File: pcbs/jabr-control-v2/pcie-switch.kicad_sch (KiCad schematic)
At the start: 27 parts, among them Q301 DMN21D2UFB-7B, U301 SYA75603A, U302 PCI11010C, Y301 XRCGB25M000F3A16R0

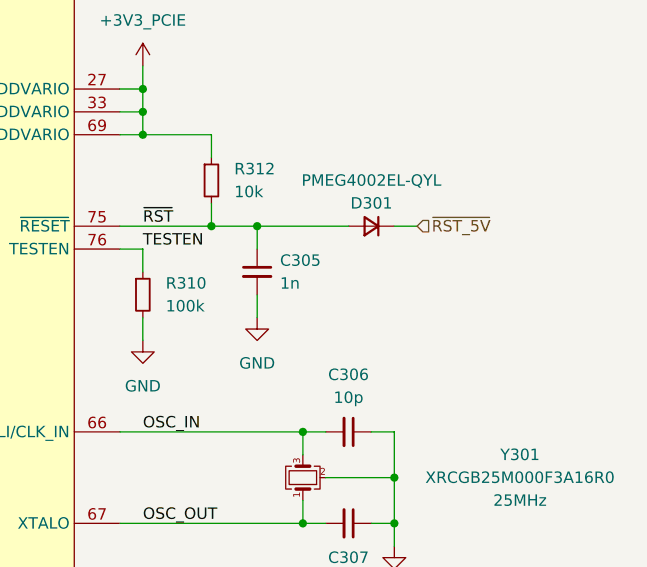
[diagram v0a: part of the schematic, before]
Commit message: Power circuitry done
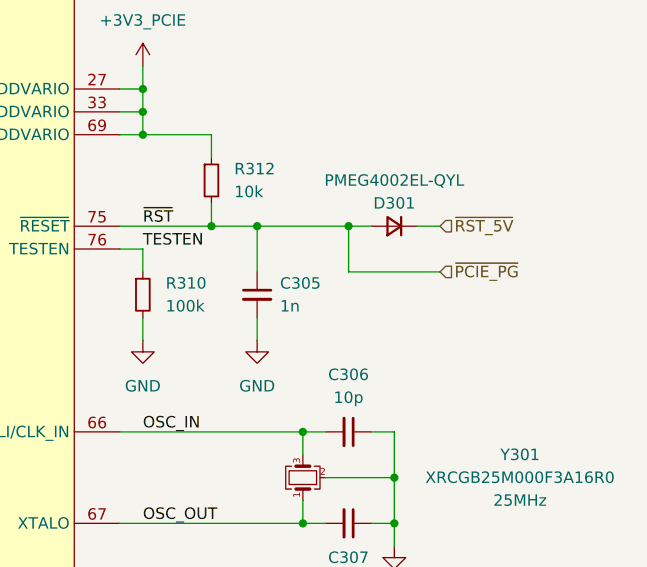
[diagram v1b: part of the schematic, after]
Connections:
- net ~{RST} renamed ~{PCIE_PG}
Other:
- moved on the sheet: C305, D301
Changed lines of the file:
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@@
 	)
 	(junction
-		(at 360.68 134.62)
+		(at 208.28 91.44)
 		(diameter 0)
 		(color 0 0 0 0)
 	)
 	(junction
-		(at 208.28 91.44)
+		(at 375.92 162.56)
 		(diameter 0)
 		(color 0 0 0 0)
 	)
 	(junction
-		(at 375.92 162.56)
+		(at 297.18 116.84)
 		(diameter 0)
 		(color 0 0 0 0)
 	)
 	(junction
-		(at 297.18 116.84)
+		(at 370.84 134.62)
 		(diameter 0)
 		(color 0 0 0 0)
@@
 	)
 	(junction
+		(at 360.68 134.62)
+		(diameter 0)
+		(color 0 0 0 0)
+	)
+	(junction
 		(at 297.18 137.16)
 		(diameter 0)
@@
 	(wire
 		(pts
-			(xy 360.68 142.24) (xy 360.68 144.78)
+			(xy 360.68 144.78) (xy 360.68 147.32)
 		)
 		(stroke
@@
 	(wire
 		(pts
+			(xy 370.84 139.7) (xy 370.84 134.62)
+		)
+		(stroke
+			(width 0)
+			(type default)
+		)
+	)
+	(wire
+		(pts
 			(xy 297.18 175.26) (xy 297.18 177.8)
 		)
@@
 	(wire
 		(pts
+			(xy 381 139.7) (xy 370.84 139.7)
+		)
+		(stroke
+			(width 0)
+			(type default)
+		)
+	)
+	(wire
+		(pts
 			(xy 347.98 101.6) (xy 347.98 104.14)
 		)
@@
 	(wire
 		(pts
-			(xy 375.92 134.62) (xy 378.46 134.62)
+			(xy 378.46 134.62) (xy 381 134.62)
 		)
 		(stroke
@@
 	(wire
 		(pts
-			(xy 360.68 134.62) (xy 360.68 137.16)
+			(xy 360.68 134.62) (xy 360.68 139.7)
 		)
 		(stroke
@@
 		)
 	)
+	(wire
+		(pts
+			(xy 370.84 134.62) (xy 373.38 134.62)
+		)
+		(stroke
+			(width 0)
+			(type default)
+		)
+	)
 	(polyline
 		(pts
@@
 	(hierarchical_label "~{RST_5V}"
 		(shape input)
-		(at 378.46 134.62 0)
+		(at 381 134.62 0)
+		(effects
+			(font
+				(size 1.27 1.27)
+			)
+			(justify left)
+		)
+	)
+	(hierarchical_label "~{PCIE_PG}"
+		(shape input)
+		(at 381 139.7 0)
 		(effects
 			(font
@@
 	(symbol
 		(lib_id "DEV:C_SMALL")
-		(at 360.68 139.7 0)
+		(at 360.68 142.24 0)
 		(unit 1)
 		(body_style 1)
@@
 		(dnp no)
 		(property "Reference" "C305"
-			(at 363.22 138.4362 0)
+			(at 363.22 140.9762 0)
 			(show_name no)
 			(do_not_autoplace no)
@@
 		)
 		(property "Value" "1n"
-			(at 363.22 140.9762 0)
+			(at 363.22 143.5162 0)
 			(show_name no)
 			(do_not_autoplace no)
@@
 		)
 		(property "Footprint" "project_footprints:C_0402"
-			(at 360.68 139.7 0)
+			(at 360.68 142.24 0)
 			(hide yes)
 			(show_name no)
@@
 		)
 		(property "Datasheet" ""
-			(at 360.68 139.7 0)
+			(at 360.68 142.24 0)
 			(hide yes)
 			(show_name no)
@@
 		)
 		(property "Description" "Unpolarized capacitor, small symbol"
-			(at 360.68 139.7 0)
+			(at 360.68 142.24 0)
 			(hide yes)
 			(show_name no)
@@
 		)
 		(property "Field6" ""
-			(at 360.68 139.7 0)
+			(at 360.68 142.24 0)
 			(hide yes)
 			(show_name no)
@@
 		)
 		(property "Field7" ""
-			(at 360.68 139.7 0)
+			(at 360.68 142.24 0)
 			(hide yes)
 			(show_name no)
@@
 		)
 		(property "Part Description" ""
-			(at 360.68 139.7 0)
+			(at 360.68 142.24 0)
 			(hide yes)
 			(show_name no)
@@
 	(symbol
 		(lib_id "power:GND")
-		(at 360.68 144.78 0)
+		(at 360.68 147.32 0)
 		(unit 1)
 		(body_style 1)
@@
 		(fields_autoplaced yes)
 		(property "Reference" "#PWR0315"
-			(at 360.68 151.13 0)
+			(at 360.68 153.67 0)
 			(hide yes)
 			(show_name no)
@@
 		)
 		(property "Value" "GND"
-			(at 360.68 149.86 0)
+			(at 360.68 152.4 0)
 			(show_name no)
 			(do_not_autoplace no)
@@
 		)
 		(property "Footprint" ""
-			(at 360.68 144.78 0)
+			(at 360.68 147.32 0)
 			(hide yes)
 			(show_name no)
@@
 		)
 		(property "Datasheet" ""
-			(at 360.68 144.78 0)
+			(at 360.68 147.32 0)
 			(hide yes)
 			(show_name no)
@@
 		)
 		(property "Description" "Power symbol creates a global label with name \"GND\" , ground"
-			(at 360.68 144.78 0)
+			(at 360.68 147.32 0)
 			(hide yes)
 			(show_name no)
@@
 	(symbol
 		(lib_id "DIODE:PMEG4002EL-QYL")
-		(at 373.38 134.62 0)
+		(at 375.92 134.62 0)
 		(mirror y)
 		(unit 1)
@@
 		(dnp no)
 		(property "Reference" "D301"
-			(at 373.38 132.08 0)
+			(at 375.92 132.08 0)
 			(show_name no)
 			(do_not_autoplace no)
@@
 		)
 		(property "Value" "PMEG4002EL-QYL"
-			(at 373.38 129.54 0)
+			(at 375.92 129.54 0)
 			(show_name no)
 			(do_not_autoplace no)
@@
 		)
 		(property "Footprint" "project_footprints:PMEG4002EL-QYL"
-			(at 373.38 134.62 0)
+			(at 375.92 134.62 0)
 			(hide yes)
 			(show_name no)
@@
 		)
 		(property "Datasheet" "https://assets.nexperia.com/documents/data-sheet/PMEG4002EL-Q.pdf"
-			(at 373.38 134.62 90)
+			(at 375.92 134.62 90)
 			(hide yes)
 			(show_name no)
@@
 		)
 		(property "Description" "Diode, small symbol"
-			(at 373.38 134.62 0)
+			(at 375.92 134.62 0)
 			(hide yes)
 			(show_name no)
@@
 		)
 		(property "Sim.Device" "D"
-			(at 373.38 134.62 0)
+			(at 375.92 134.62 0)
 			(hide yes)
 			(show_name no)
@@
 		)
 		(property "Sim.Pins" "1=K 2=A"
-			(at 373.38 134.62 0)
+			(at 375.92 134.62 0)
 			(hide yes)
 			(show_name no)
@@
 		)
 		(property "Field6" ""
-			(at 373.38 134.62 0)
+			(at 375.92 134.62 0)
 			(hide yes)
 			(show_name no)
@@
 		)
 		(property "Field7" ""
-			(at 373.38 134.62 0)
+			(at 375.92 134.62 0)
 			(hide yes)
 			(show_name no)
@@
 		)
 		(property "Part Description" ""
-			(at 373.38 134.62 0)
+			(at 375.92 134.62 0)
 			(hide yes)
 			(show_name no)
